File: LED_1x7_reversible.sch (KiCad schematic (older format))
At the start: 14 parts

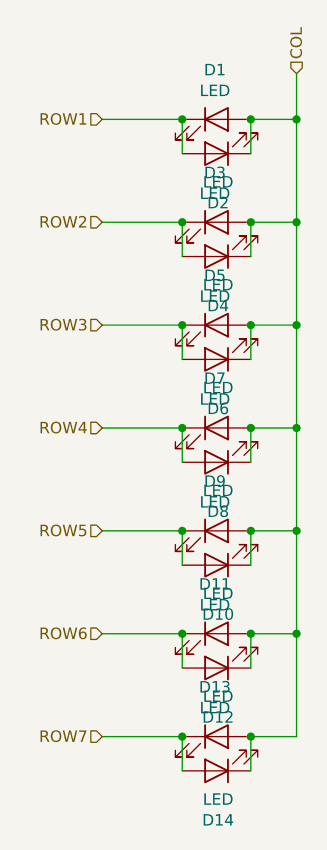
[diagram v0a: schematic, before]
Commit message: Fix matrix
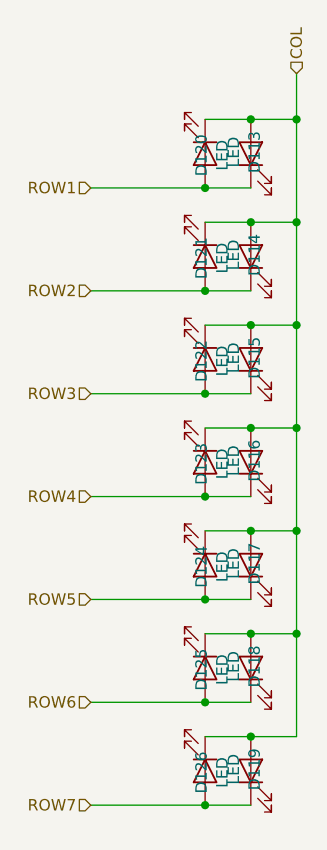
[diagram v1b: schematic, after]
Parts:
- removed D8: LED, LED_SMD:LED_0805_2012Metric, symbol Device:LED
- added D2: LED, LED_SMD:LED_0805_2012Metric, symbol Device:LED
- renumbered D2 to D8
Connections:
- net COL: now also D1.1 (K), D10.2 (A), D12.2 (A), D14.2 (A), D3.1 (K), D5.1 (K), D7.1 (K), D8.2 (A), D2.1 (K); no longer D1.2 (A), D10.1 (K), D12.1 (K), D14.1 (K), D3.2 (A), D5.2 (A), D7.2 (A), D8.1 (K)
- net ROW1: now also D1.2 (A), D8.1 (K); no longer D1.1 (K), D8.2 (A)
- net ROW2: now also D9.1 (K), D2.2 (A); no longer D3.1 (K), D4.2 (A)
- net ROW3: now also D10.1 (K), D3.2 (A); no longer D5.1 (K), D6.2 (A)
- net ROW4: now also D11.1 (K), D4.2 (A); no longer D7.1 (K)
- net ROW5: now also D12.1 (K), D5.2 (A); no longer D10.2 (A), D9.1 (K)
- net ROW6: now also D13.1 (K), D6.2 (A); no longer D11.1 (K), D12.2 (A)
- net ROW7: now also D14.1 (K), D7.2 (A); no longer D13.1 (K), D14.2 (A)
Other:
- moved on the sheet: D113, D120
